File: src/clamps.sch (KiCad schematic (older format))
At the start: 38 parts, among them P1 CONN_01X12, U1 LM741, U2 LM741, U3 LM741, U4 LM741, U5 LM741, U6 LM741

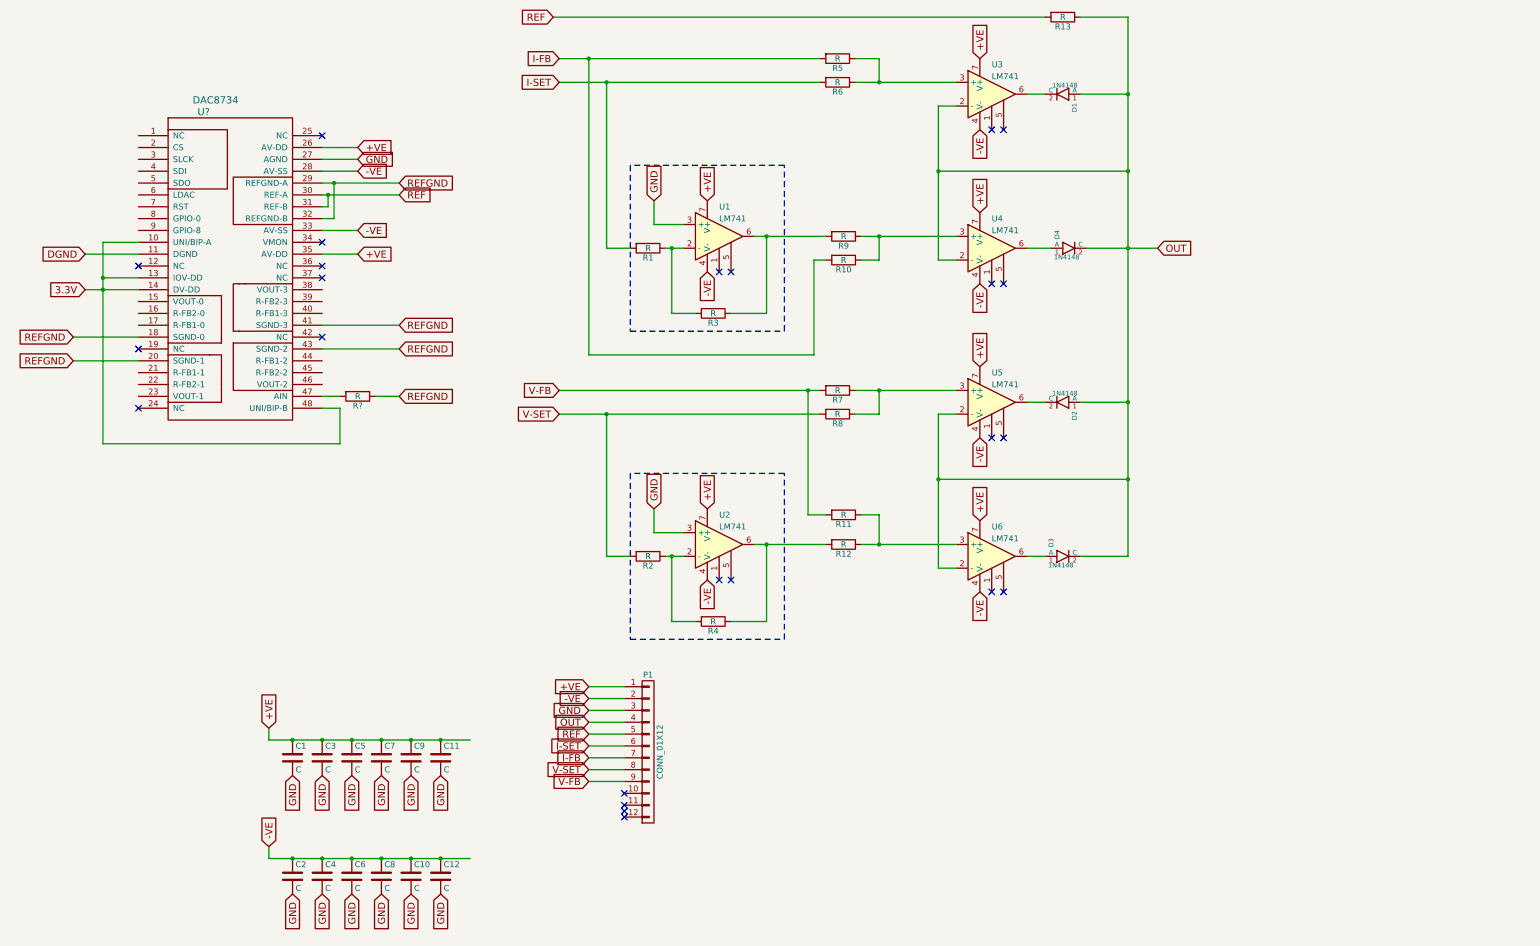
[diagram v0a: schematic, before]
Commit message: update
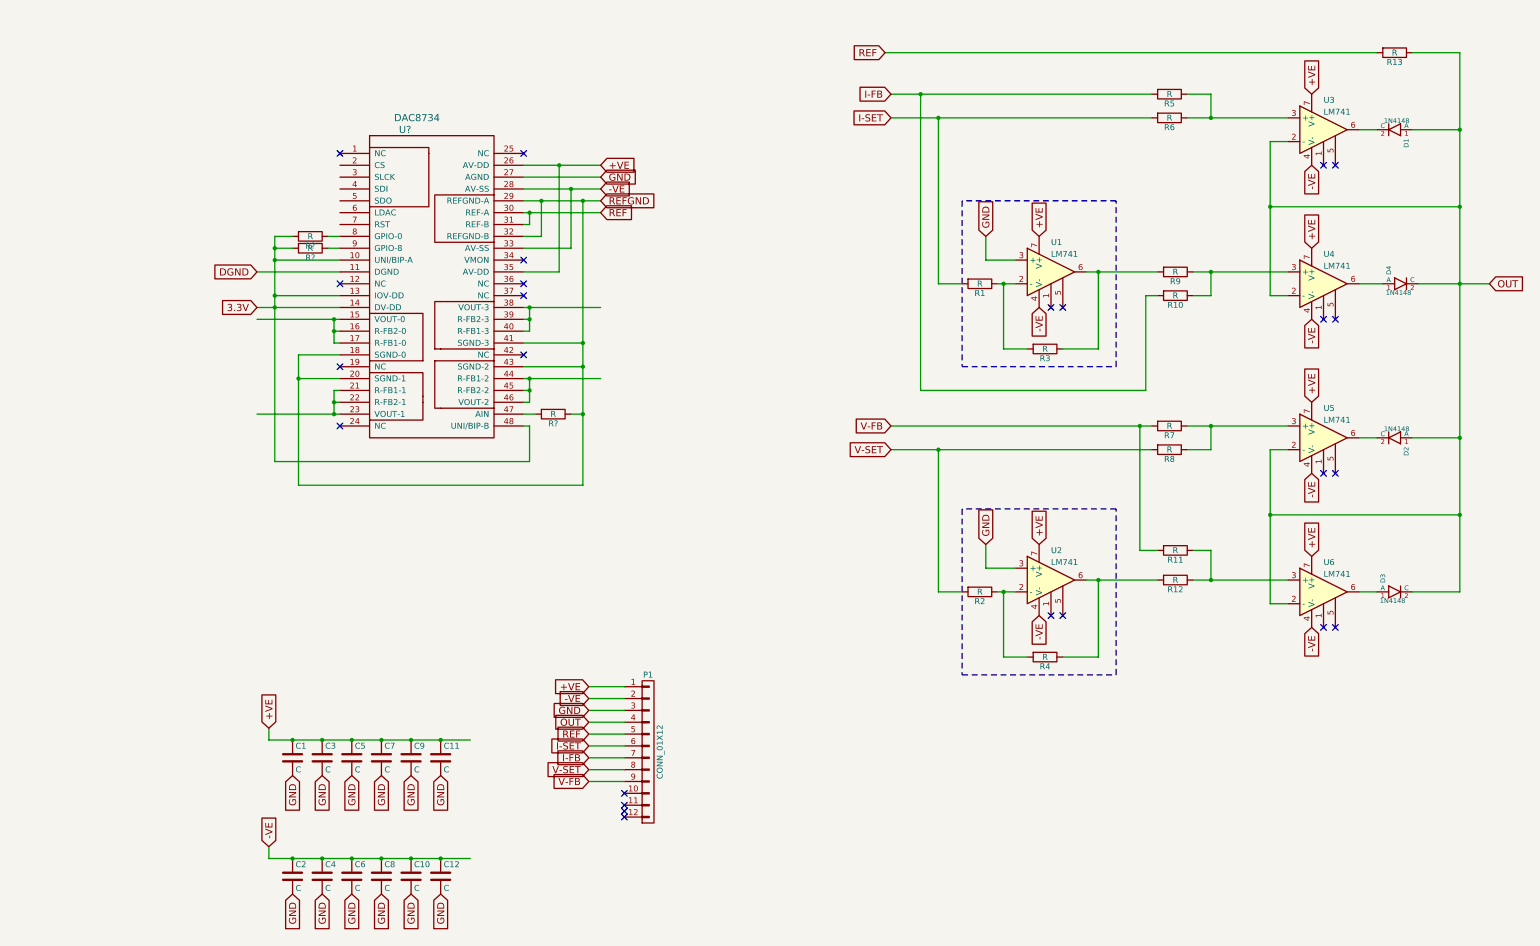
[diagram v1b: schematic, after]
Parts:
- added R? (x2): R, symbol R
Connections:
- wire segments 99 -> 178
- no-connect marks 24 -> 25
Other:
- moved on the sheet: D1, D2, D3, D4, R1, R10, R11, R12, R13, R2, R3, R4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
